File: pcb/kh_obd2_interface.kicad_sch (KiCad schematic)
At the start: 0 parts

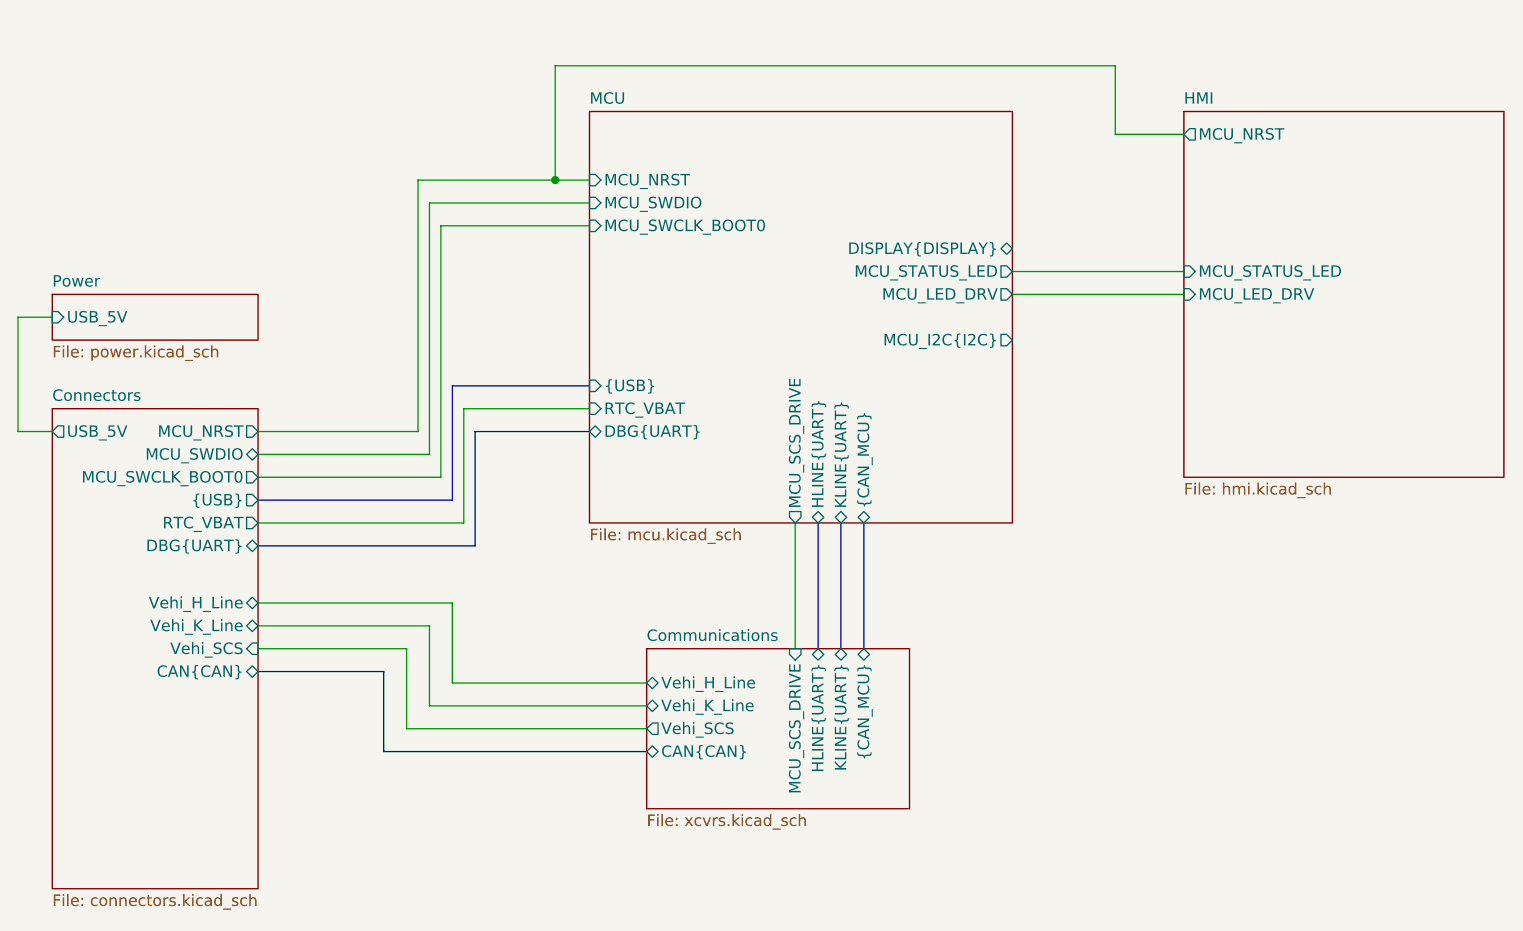
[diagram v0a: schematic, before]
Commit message: connector prep
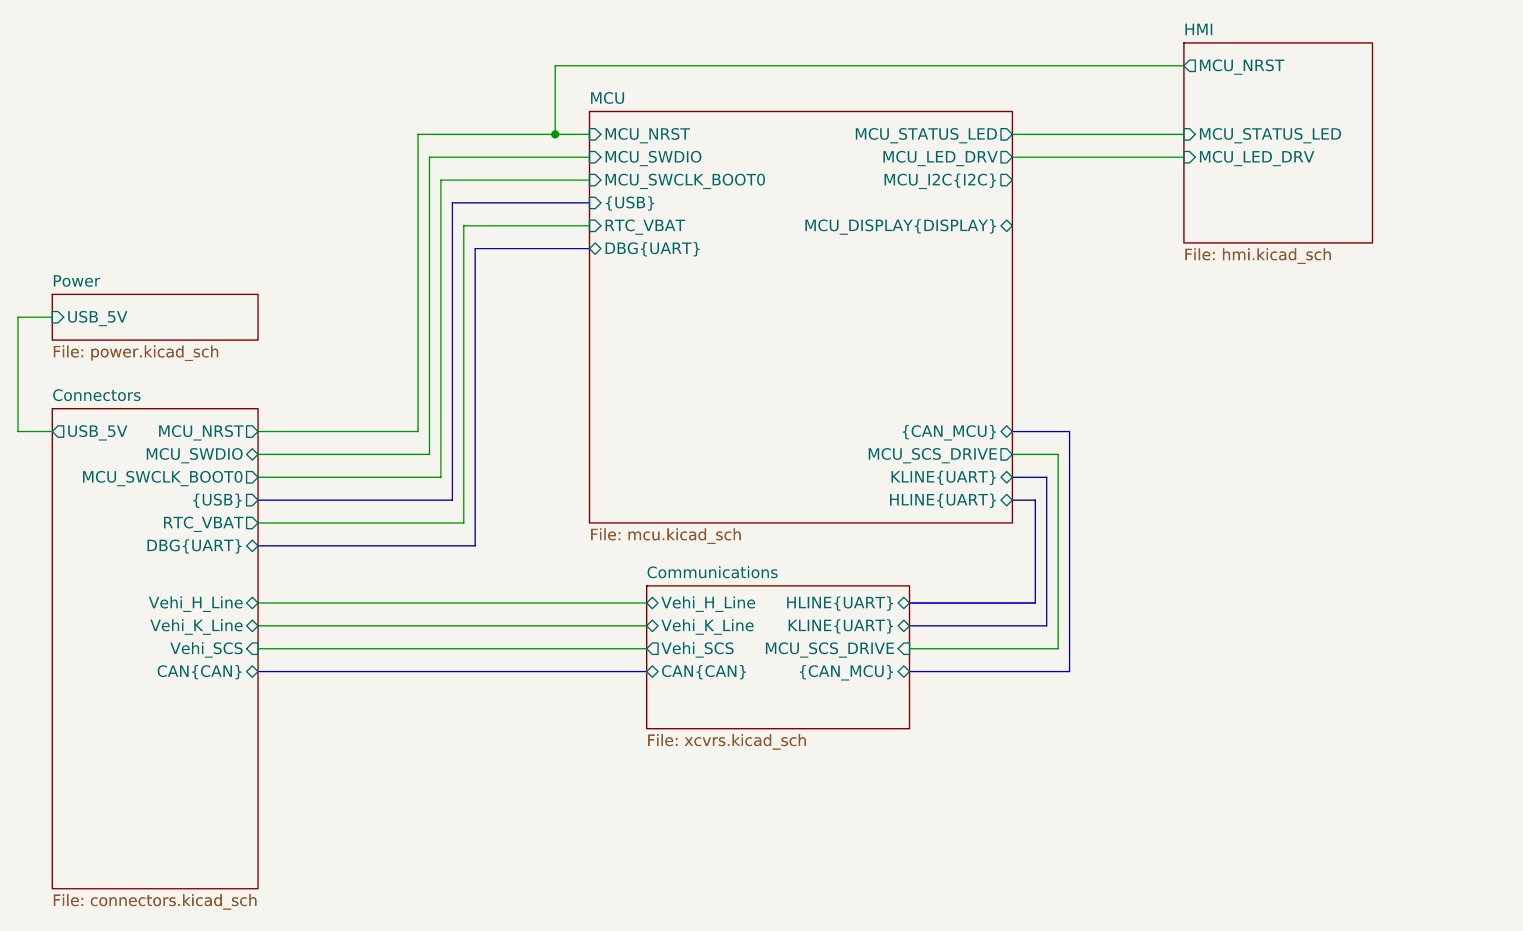
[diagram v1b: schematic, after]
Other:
- sheet MCU ports: added MCU_DISPLAY{DISPLAY}; removed DISPLAY{DISPLAY}
